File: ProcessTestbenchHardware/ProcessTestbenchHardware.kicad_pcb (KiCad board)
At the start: 2 copper layers, 104 x 63 mm, 54 parts, among them J1 Fluxo1, J11 LSLL1, J12 LSHH2, J13 LSLL2, J2 Fluxo2, J3 Fluxo, J4 Pressao1, J5 Pressao2, J6 Term1, J7 Term2, J8 LSHH1, Q1 IRLZ44N, Q2 IRLZ44N, Q3 IRLZ44N, Q4 IRLZ44N, Q5 IRLZ44N, U2 MAX485E

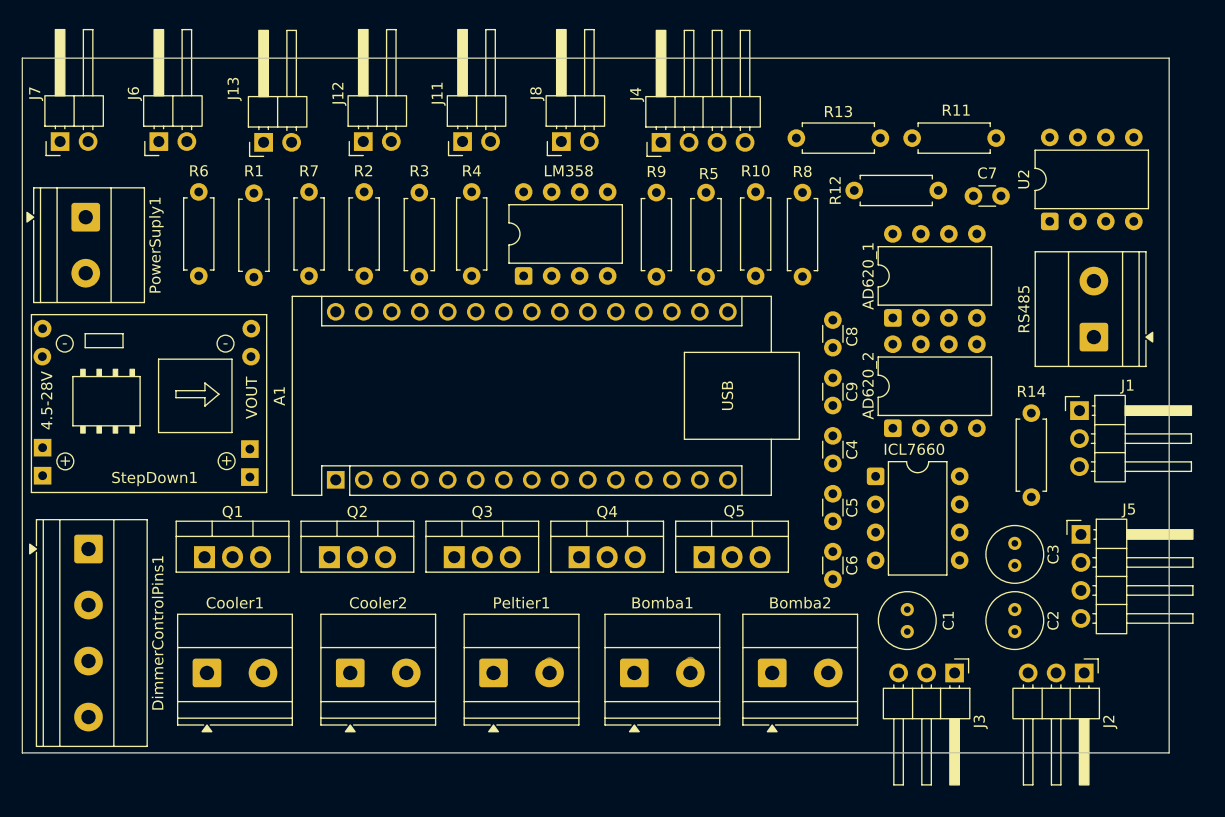
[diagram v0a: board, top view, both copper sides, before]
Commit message: PCB routing
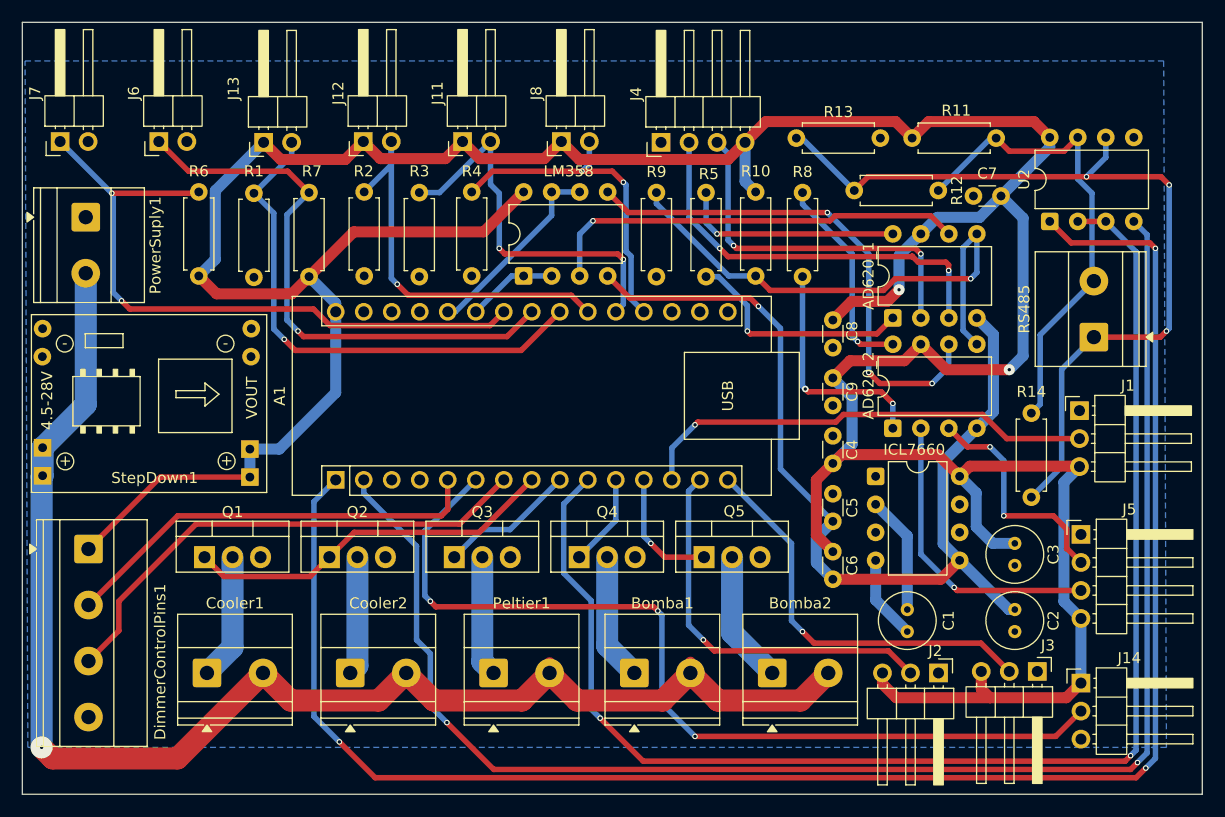
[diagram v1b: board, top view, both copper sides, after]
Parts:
- added J14: Servo, Connector_PinHeader_2.54mm:PinHeader_1x03_P2.54mm_Horizontal, F.Cu at (153.5, 106.4)
- J3: value Fluxo -> Fluxo3
- moved J2 13.2 mm to (140.6, 105.5)
- moved R7 7.68 mm to (83.5, 69.6), turned to 90 degrees
- moved R12 7.62 mm to (140.6, 61.8), turned to 180 degrees
- moved J3 7.50 mm to (149.5, 105.4)
- moved C8 2.50 mm to (131.0, 76.0), turned to 90 degrees
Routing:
- net +5V: track 0.00 -> 333.3 mm, vias 0 -> 2
- net /MAX485_RX: track 0.00 -> 158.4 mm, vias 0 -> 3
- net /MAX485_TX: track 0.00 -> 139.7 mm, vias 0 -> 2
- net +12V: track 5.01 -> 132.9 mm, vias 0 -> 1
- net /DE/RE_MAX485: track 0.00 -> 126.1 mm, vias 0 -> 2
- net -5V: track 0.00 -> 87.8 mm, vias 0 -> 1
- net /SaidaServoMotor: track 0.00 -> 82.8 mm, vias 0 -> 3
- net Net-(RS485-Pin_1): track 0.00 -> 77.9 mm, vias 0 -> 3
- net /AnalogTemp2: track 0.00 -> 60.8 mm, vias 0 -> 2
- net /AnalogTemp1: track 0.00 -> 51.7 mm, vias 0 -> 1
- net /AD620Ref: track 0.00 -> 48.5 mm, vias 0 -> 1
- net /LSLL2: track 0.00 -> 48.1 mm, vias 0 -> 1
- net Net-(LM358B-+): track 0.00 -> 47.1 mm, vias 0 -> 3
- net /DimmerControl: track 0.00 -> 46.0 mm
- net Net-(RS485-Pin_2): track 0.00 -> 43.6 mm
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- added copper zone on B.Cu, net GND
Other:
- board size 104 x 63 mm -> 107 x 70 mm
